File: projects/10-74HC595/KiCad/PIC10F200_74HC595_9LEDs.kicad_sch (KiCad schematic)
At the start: 21 parts, among them U1 PIC10F200-IP, U2 74HC595

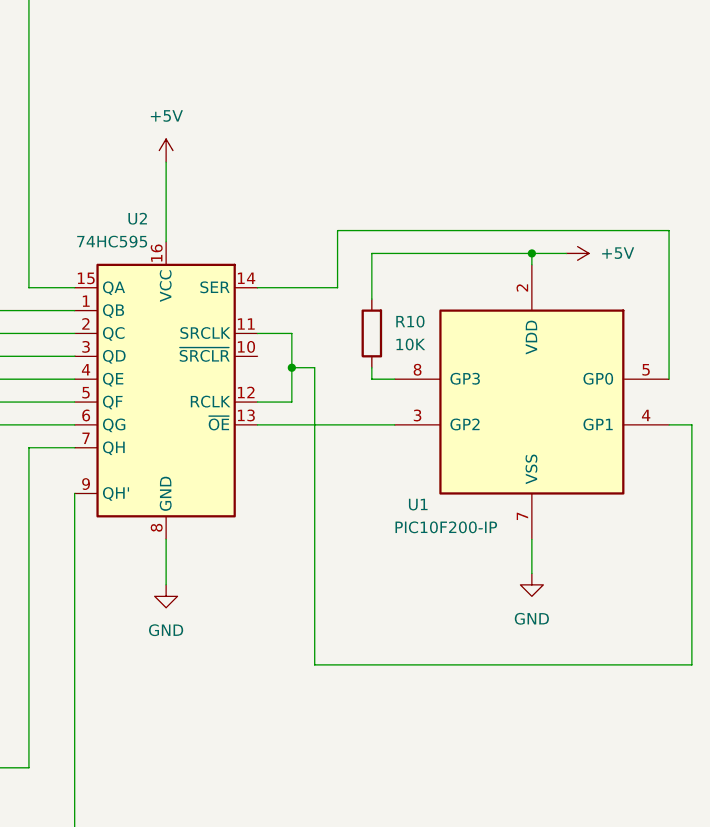
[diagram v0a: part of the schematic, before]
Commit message: Doc
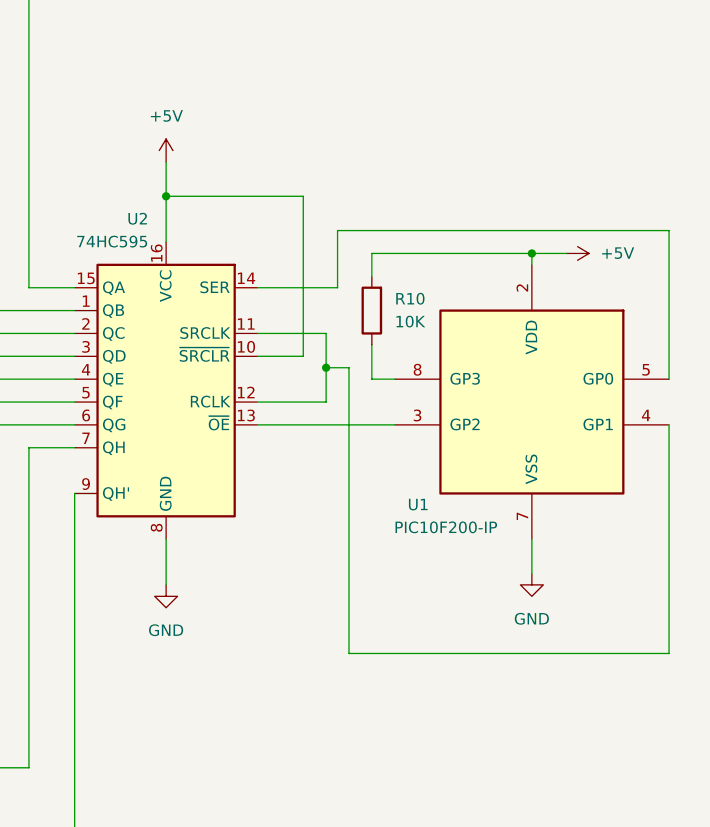
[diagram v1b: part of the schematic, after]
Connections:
- net +5V: now also U2.10 (~{SRCLR})
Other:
- moved on the sheet: R10
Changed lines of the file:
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@@
   (junction (at 80.01 129.54) (diameter 0) (color 0 0 0 0)
   )
+  (junction (at 160.02 97.79) (diameter 0) (color 0 0 0 0)
+  )
   (junction (at 182.88 85.09) (diameter 0) (color 0 0 0 0)
   )
@@
   (junction (at 80.01 76.2) (diameter 0) (color 0 0 0 0)
   )
-  (junction (at 156.21 97.79) (diameter 0) (color 0 0 0 0)
+  (junction (at 142.24 78.74) (diameter 0) (color 0 0 0 0)
   )
   (wire (pts (xy 87.63 115.57) (xy 96.52 115.57))
@@
     (stroke (width 0) (type default))
   )
-  (wire (pts (xy 156.21 97.79) (xy 156.21 101.6))
-    (stroke (width 0) (type default))
-  )
   (wire (pts (xy 152.4 104.14) (xy 167.64 104.14))
     (stroke (width 0) (type default))
   )
-  (wire (pts (xy 156.21 101.6) (xy 152.4 101.6))
-    (stroke (width 0) (type default))
-  )
   (wire (pts (xy 104.14 142.24) (xy 127 142.24))
     (stroke (width 0) (type default))
@@
     (stroke (width 0) (type default))
   )
-  (wire (pts (xy 152.4 93.98) (xy 156.21 93.98))
-    (stroke (width 0) (type default))
-  )
   (wire (pts (xy 182.88 116.84) (xy 182.88 120.65))
     (stroke (width 0) (type default))
@@
     (stroke (width 0) (type default))
   )
+  (wire (pts (xy 152.4 93.98) (xy 160.02 93.98))
+    (stroke (width 0) (type default))
+  )
+  (wire (pts (xy 152.4 96.52) (xy 157.48 96.52))
+    (stroke (width 0) (type default))
+  )
   (wire (pts (xy 80.01 76.2) (xy 80.01 88.9))
     (stroke (width 0) (type default))
   )
+  (wire (pts (xy 142.24 78.74) (xy 157.48 78.74))
+    (stroke (width 0) (type default))
+  )
   (wire (pts (xy 132.08 99.06) (xy 118.11 99.06))
     (stroke (width 0) (type default))
@@
     (stroke (width 0) (type default))
   )
-  (wire (pts (xy 200.66 104.14) (xy 200.66 130.81))
-    (stroke (width 0) (type default))
-  )
   (wire (pts (xy 120.65 93.98) (xy 120.65 76.2))
     (stroke (width 0) (type default))
@@
     (stroke (width 0) (type default))
   )
-  (wire (pts (xy 156.21 93.98) (xy 156.21 97.79))
-    (stroke (width 0) (type default))
-  )
   (wire (pts (xy 132.08 111.76) (xy 132.08 157.48))
     (stroke (width 0) (type default))
@@
     (stroke (width 0) (type default))
   )
+  (wire (pts (xy 142.24 78.74) (xy 142.24 83.82))
+    (stroke (width 0) (type default))
+  )
   (wire (pts (xy 118.11 88.9) (xy 104.14 88.9))
     (stroke (width 0) (type default))
@@
     (stroke (width 0) (type default))
   )
-  (wire (pts (xy 158.75 130.81) (xy 158.75 97.79))
-    (stroke (width 0) (type default))
-  )
   (wire (pts (xy 132.08 91.44) (xy 123.19 91.44))
     (stroke (width 0) (type default))
@@
     (stroke (width 0) (type default))
   )
-  (wire (pts (xy 142.24 74.93) (xy 142.24 83.82))
-    (stroke (width 0) (type default))
-  )
-  (wire (pts (xy 165.1 97.79) (xy 165.1 99.06))
+  (wire (pts (xy 142.24 74.93) (xy 142.24 78.74))
+    (stroke (width 0) (type default))
+  )
+  (wire (pts (xy 157.48 96.52) (xy 157.48 78.74))
+    (stroke (width 0) (type default))
+  )
+  (wire (pts (xy 160.02 93.98) (xy 160.02 97.79))
+    (stroke (width 0) (type default))
+  )
+  (wire (pts (xy 165.1 95.25) (xy 165.1 99.06))
     (stroke (width 0) (type default))
   )
@@
     (stroke (width 0) (type default))
   )
+  (wire (pts (xy 152.4 101.6) (xy 160.02 101.6))
+    (stroke (width 0) (type default))
+  )
   (wire (pts (xy 104.14 157.48) (xy 132.08 157.48))
     (stroke (width 0) (type default))
   )
+  (wire (pts (xy 162.56 97.79) (xy 160.02 97.79))
+    (stroke (width 0) (type default))
+  )
+  (wire (pts (xy 162.56 129.54) (xy 162.56 97.79))
+    (stroke (width 0) (type default))
+  )
   (wire (pts (xy 132.08 93.98) (xy 120.65 93.98))
     (stroke (width 0) (type default))
@@
     (stroke (width 0) (type default))
   )
-  (wire (pts (xy 198.12 104.14) (xy 200.66 104.14))
-    (stroke (width 0) (type default))
-  )
-  (wire (pts (xy 165.1 90.17) (xy 165.1 85.09))
+  (wire (pts (xy 165.1 87.63) (xy 165.1 85.09))
     (stroke (width 0) (type default))
   )
@@
     (stroke (width 0) (type default))
   )
-  (wire (pts (xy 200.66 130.81) (xy 158.75 130.81))
+  (wire (pts (xy 160.02 97.79) (xy 160.02 101.6))
+    (stroke (width 0) (type default))
+  )
+  (wire (pts (xy 198.12 129.54) (xy 162.56 129.54))
     (stroke (width 0) (type default))
   )
@@
     (stroke (width 0) (type default))
   )
+  (wire (pts (xy 198.12 104.14) (xy 198.12 129.54))
+    (stroke (width 0) (type default))
+  )
   (wire (pts (xy 120.65 76.2) (xy 104.14 76.2))
-    (stroke (width 0) (type default))
-  )
-  (wire (pts (xy 158.75 97.79) (xy 156.21 97.79))
     (stroke (width 0) (type default))
   )
@@
     )
   )
-  (symbol (lib_id "Device:R") (at 165.1 93.98 180) (unit 1)
-    (in_bom yes) (on_board yes) (dnp no) (fields_autoplaced)
-    (property "Reference" "R10" (at 167.64 92.71 0)
+  (symbol (lib_id "Device:R") (at 165.1 91.44 180) (unit 1)
+    (in_bom yes) (on_board yes) (dnp no) (fields_autoplaced)
+    (property "Reference" "R10" (at 167.64 90.17 0)
       (effects (font (size 1.27 1.27)) (justify right))
     )
-    (property "Value" "10K" (at 167.64 95.25 0)
+    (property "Value" "10K" (at 167.64 92.71 0)
       (effects (font (size 1.27 1.27)) (justify right))
     )
-    (property "Footprint" "" (at 166.878 93.98 90)
-      (effects (font (size 1.27 1.27)) hide)
-    )
-    (property "Datasheet" "~" (at 165.1 93.98 0)
-      (effects (font (size 1.27 1.27)) hide)
-    )
+    (property "Footprint" "" (at 166.878 91.44 90)
+      (effects (font (size 1.27 1.27)) hide)
+    )
+    (property "Datasheet" "~" (at 165.1 91.44 0)
+      (effects (font (size 1.27 1.27)) hide)
+    )

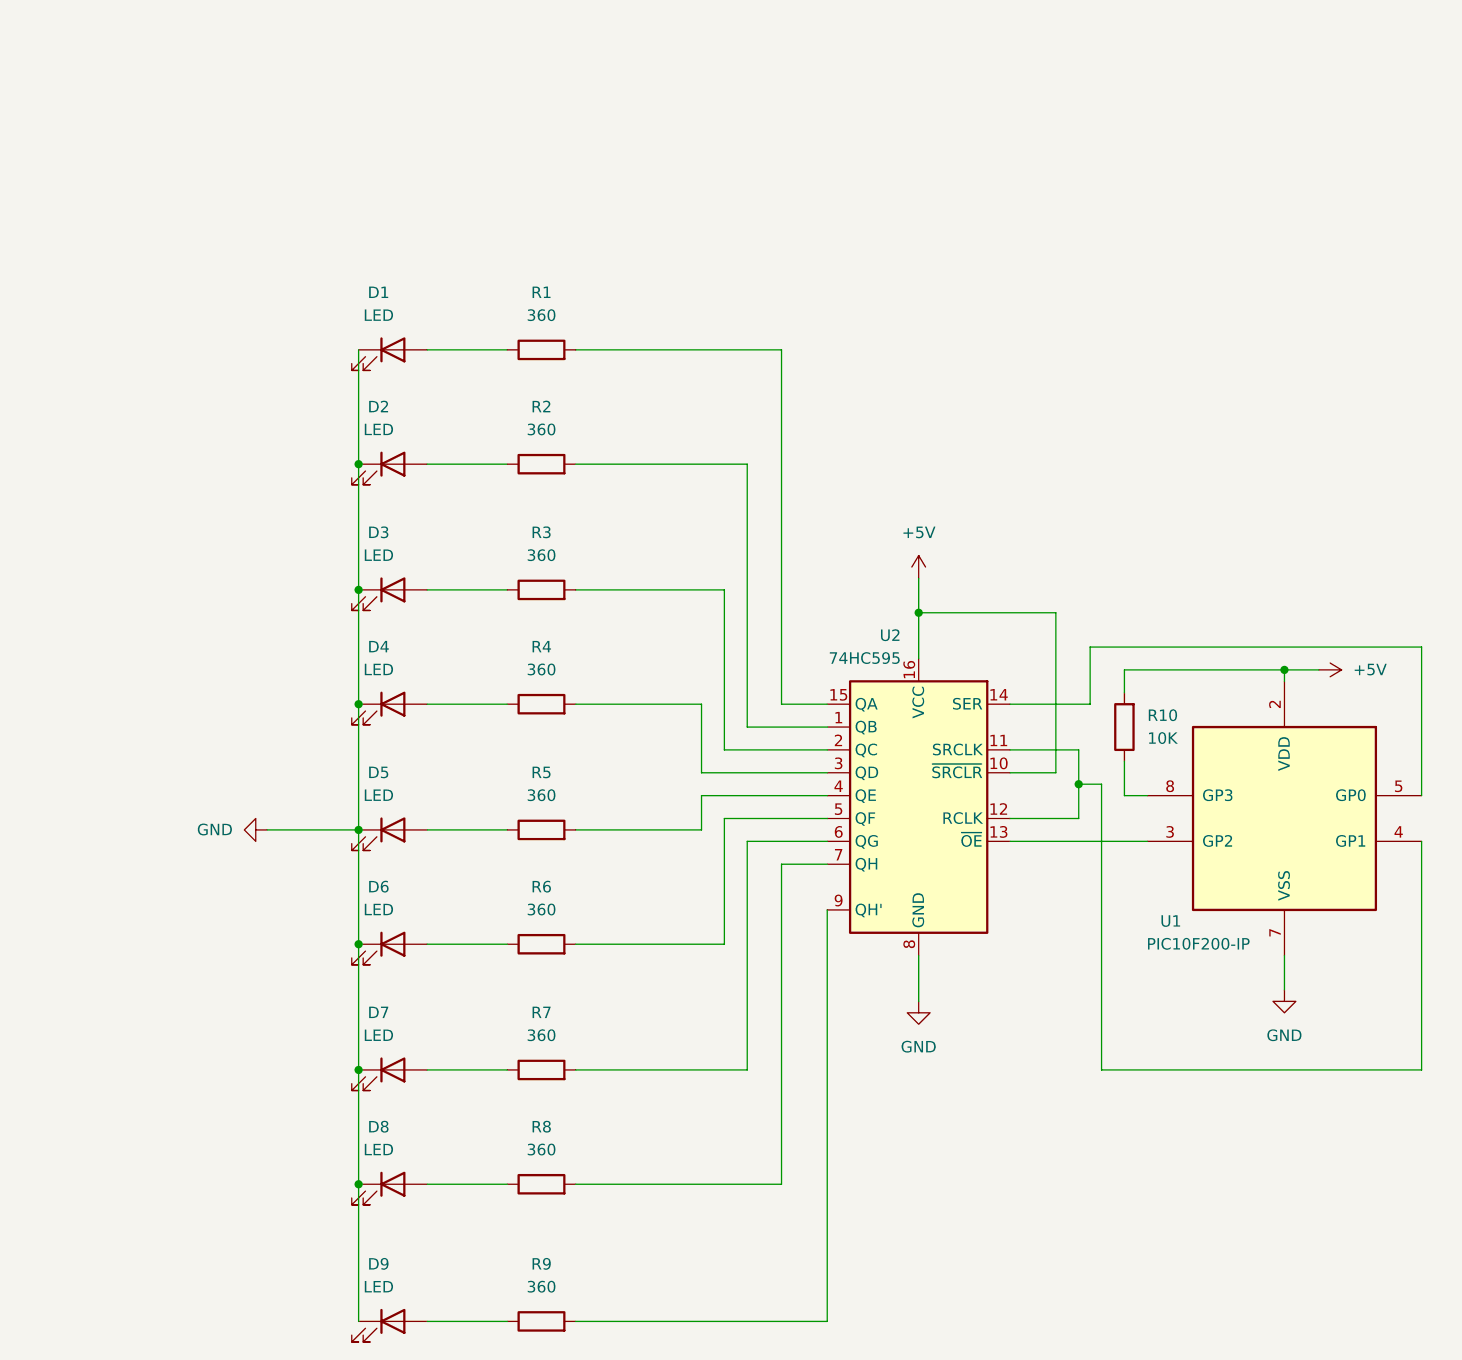
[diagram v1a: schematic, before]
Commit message: Documentation
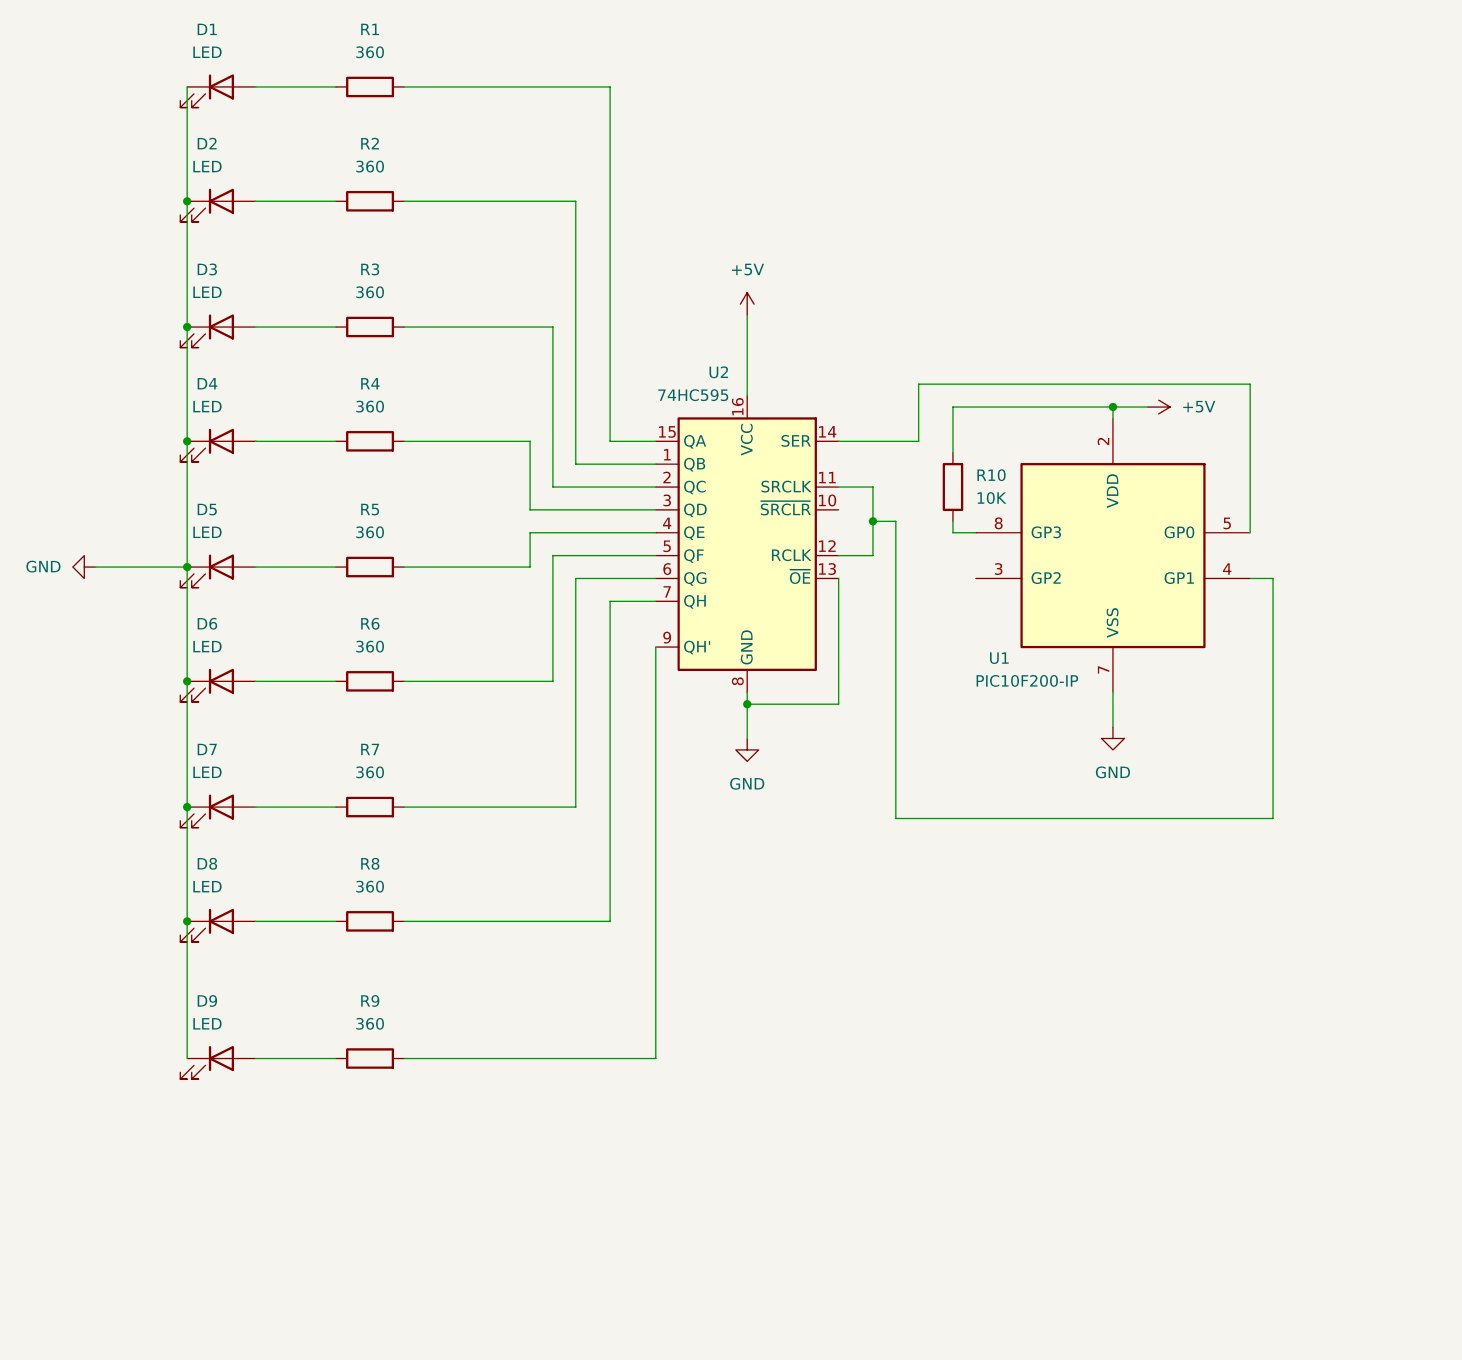
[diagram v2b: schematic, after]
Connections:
- net +5V: no longer U2.10 (~{SRCLR})
- net GND: now also U2.13 (~{OE})
- net at U1.3 (GP2): no longer U2.13 (~{OE})
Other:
- title: PIC10F200 and 74HC595 setup -> PIC10F200 and 74HC595 two wires setup
- moved on the sheet: D1, D2, D3, D4, D5, D6, D7, D8, D9, R1, R10, R2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
